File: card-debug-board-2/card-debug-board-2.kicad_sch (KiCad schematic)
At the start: 29 parts, among them J1 2-1734592-0, J2 Conn_01x05, J5 0676430910, J6 629105150521, SW1 PCM13SMTR, SW2 B3F-1000, SW5 210-2LPS, U1 MIC5205-3.3YM5

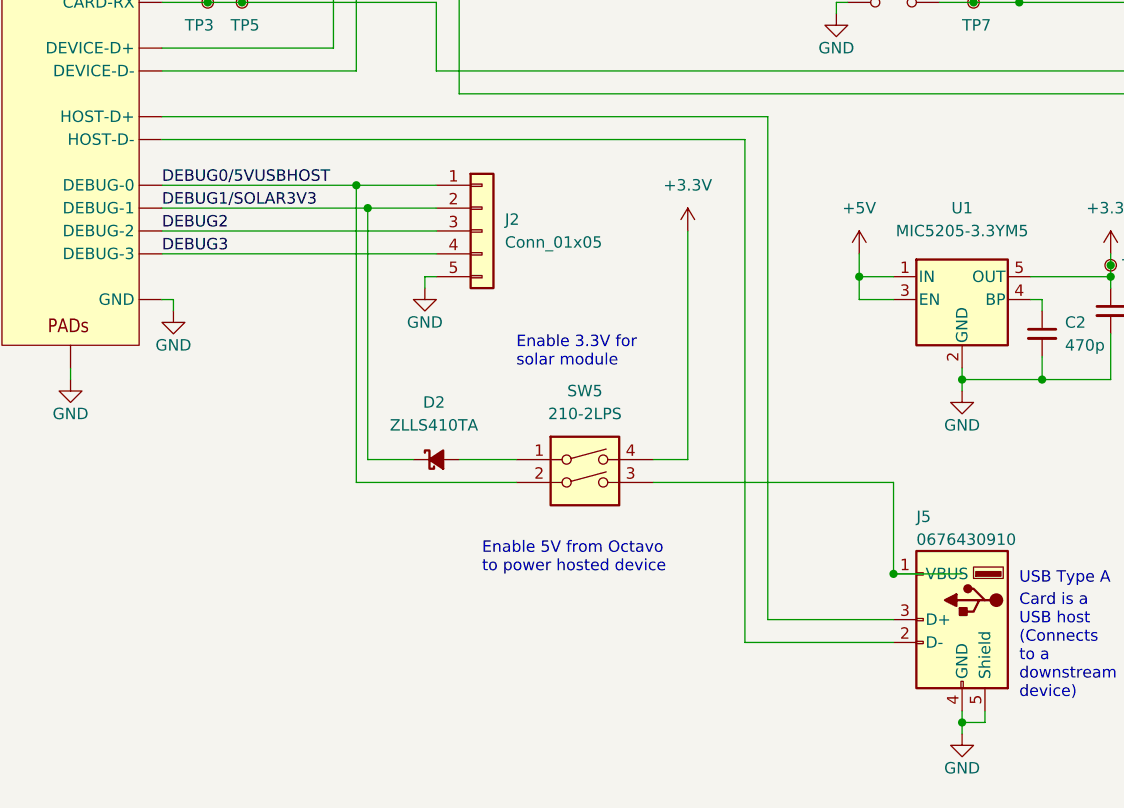
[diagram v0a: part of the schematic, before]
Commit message: restore v2 card debug board files
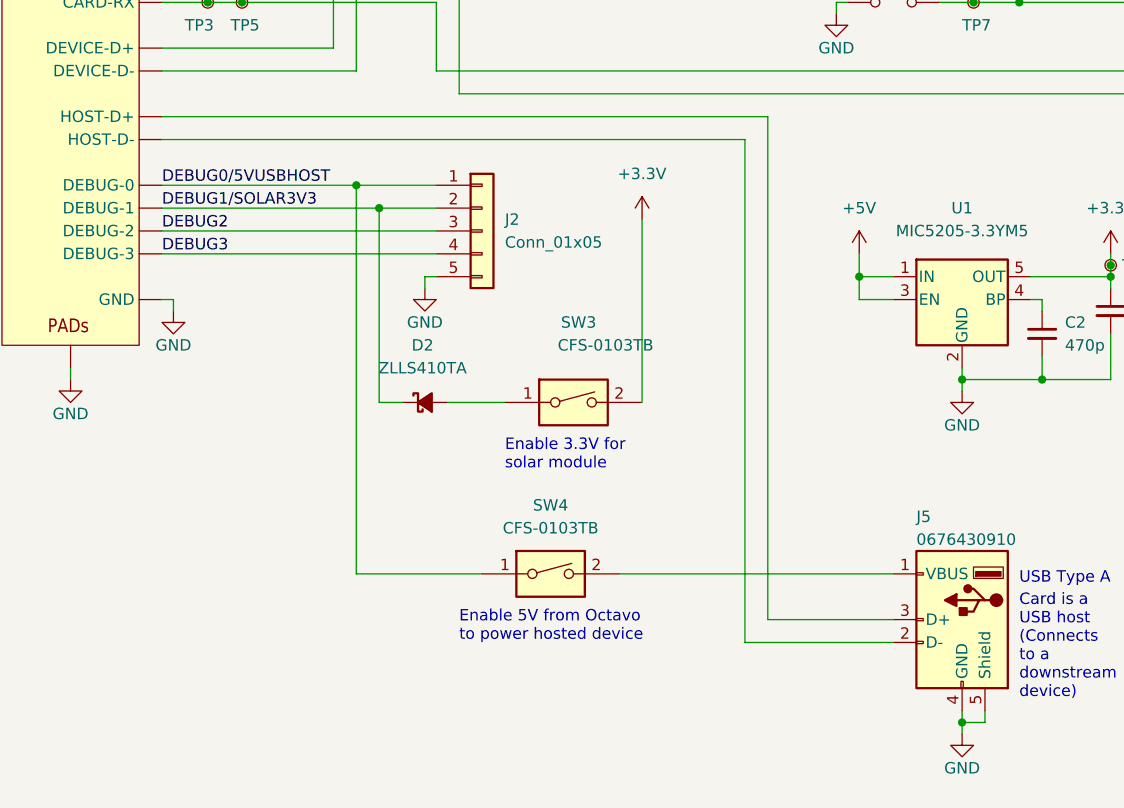
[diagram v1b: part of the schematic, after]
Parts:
- removed SW5: 210-2LPS, Button_Switch_THT:SW_DIP_SPSTx02_Slide_6.7x6.64mm_W7.62mm_P2.54mm_LowProfile, symbol Switch:SW_DIP_x02
- added SW3, SW4: CFS-0103TB, Button_Switch_SMD:SW_DIP_SPSTx01_Slide_Copal_CHS-01B_W7.62mm_P1.27mm, symbol Switch:SW_DIP_x01
- J1: value 2-1734592-0 -> 2-1734592-0
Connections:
- net +3.3V: now also SW3.2
- net DEBUG0/5VUSBHOST: now also SW4.1
- net at D2.2 (A): now also SW3.1
- net at J5.1 (VBUS): now also SW4.2
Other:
- moved on the sheet: D2
